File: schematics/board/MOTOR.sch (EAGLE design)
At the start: 77 parts

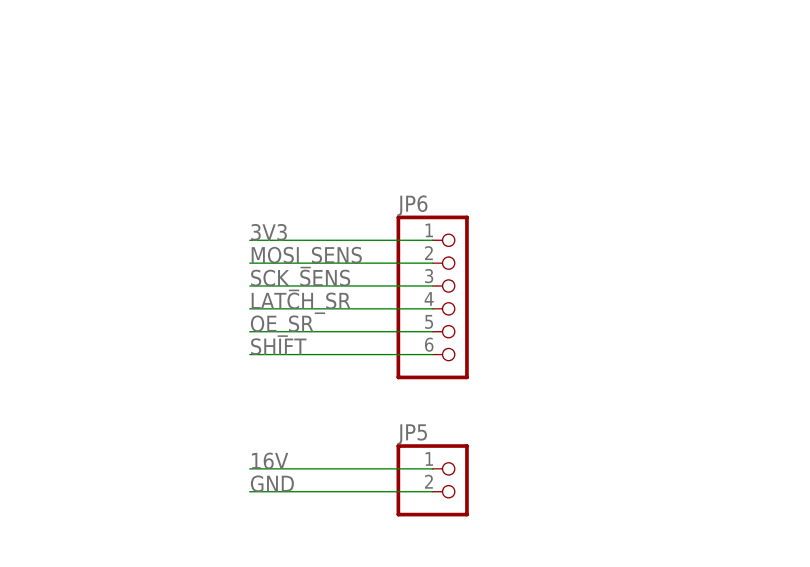
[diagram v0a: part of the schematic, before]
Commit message: Моторчики
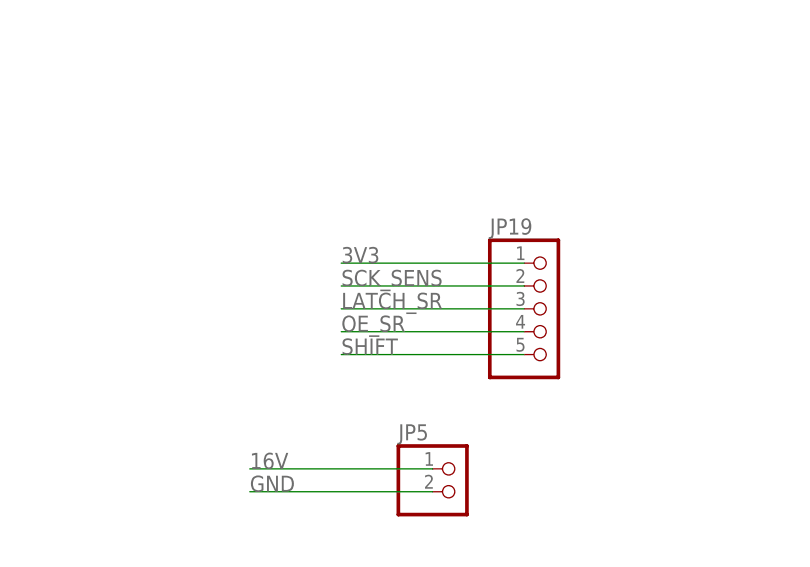
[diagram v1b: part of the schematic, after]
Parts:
- removed JP6: (no value), pinhead:PINHD-1X6
- added JP19: (no value), pinhead:PINHD-1X5
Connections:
- removed net MOSI_SENS: JP6.2
- net 3V3: now also JP19.1; no longer JP6.1
- net LATCH_SR: now also JP19.3; no longer JP6.4
- net OE_SR: now also JP19.4; no longer JP6.5
- net SCK_SENS: now also JP19.2; no longer JP6.3
- net SHIFT: now also JP19.5; no longer JP6.6
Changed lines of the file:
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@@
 <part name="U$2" library="CanCubeSat" deviceset="CONCEVIC" device=""/>
 <part name="JP5" library="pinhead" library_urn="urn:adsk.eagle:library:325" deviceset="PINHD-1X2" device="" package3d_urn="urn:adsk.eagle:package:22435/2"/>
-<part name="JP6" library="pinhead" library_urn="urn:adsk.eagle:library:325" deviceset="PINHD-1X6" device="" package3d_urn="urn:adsk.eagle:package:22472/2"/>
 <part name="SI2302CDS5" library="CanCubeSat" deviceset="SI2302CDS" device=""/>
 <part name="R7" library="rcl" library_urn="urn:adsk.eagle:library:334" deviceset="R-US_" device="R0603" package3d_urn="urn:adsk.eagle:package:23555/3" value="100R"/>
@@
 <part name="U$9" library="UNKNOWN-2024" deviceset="LOGO" device="PCB-&quot;&quot;" value="Плата МОТОРОВ"/>
 <part name="U$10" library="UNKNOWN-2024" deviceset="MOLEX-2-1.25" device=""/>
+<part name="JP19" library="pinhead" library_urn="urn:adsk.eagle:library:325" deviceset="PINHD-1X5" device="" package3d_urn="urn:adsk.eagle:package:22469/2"/>
 </parts>
 <sheets>
@@
 <attribute name="VALUE" x="-21.59" y="38.1" size="1.778" layer="96"/>
 </instance>
-<instance part="JP6" gate="A" x="-15.24" y="63.5" smashed="yes">
-<attribute name="NAME" x="-21.59" y="74.295" size="1.778" layer="95"/>
-<attribute name="VALUE" x="-21.59" y="53.34" size="1.778" layer="96"/>
-</instance>
 <instance part="SI2302CDS5" gate="G$1" x="81.28" y="-30.48" smashed="yes"/>
 <instance part="R7" gate="G$1" x="81.28" y="2.54" smashed="yes" rot="R270">
@@
 <attribute name="VALUE" x="-154.94" y="-39.37" size="1.778" layer="96" rot="R90"/>
 <attribute name="NAME" x="-165.862" y="-39.37" size="1.778" layer="95" rot="R90"/>
+</instance>
+<instance part="JP19" gate="A" x="-5.08" y="63.5" smashed="yes">
+<attribute name="NAME" x="-11.43" y="71.755" size="1.778" layer="95"/>
+<attribute name="VALUE" x="-11.43" y="53.34" size="1.778" layer="96"/>
 </instance>
 </instances>
@@
 </segment>
 <segment>
-<wire x1="-17.78" y1="71.12" x2="-38.1" y2="71.12" width="0.1524" layer="91"/>
-<label x="-38.1" y="71.12" size="1.778" layer="95"/>
-<pinref part="JP6" gate="A" pin="1"/>
+<wire x1="-7.62" y1="68.58" x2="-27.94" y2="68.58" width="0.1524" layer="91"/>
+<label x="-27.94" y="68.58" size="1.778" layer="95"/>
+<pinref part="JP19" gate="A" pin="1"/>
 </segment>
 </net>
@@
 </segment>
 <segment>
-<wire x1="-17.78" y1="60.96" x2="-38.1" y2="60.96" width="0.1524" layer="91"/>
-<label x="-38.1" y="60.96" size="1.778" layer="95"/>
-<pinref part="JP6" gate="A" pin="5"/>
+<wire x1="-7.62" y1="60.96" x2="-27.94" y2="60.96" width="0.1524" layer="91"/>
+<label x="-27.94" y="60.96" size="1.778" layer="95"/>
+<pinref part="JP19" gate="A" pin="4"/>
 </segment>
 </net>
@@
 </segment>
 </net>
-<net name="MOSI_SENS" class="0">
-<segment>
-<wire x1="-17.78" y1="68.58" x2="-38.1" y2="68.58" width="0.1524" layer="91"/>
-<label x="-38.1" y="68.58" size="1.778" layer="95"/>
-<pinref part="JP6" gate="A" pin="2"/>
-</segment>
-</net>
 <net name="SCK_SENS" class="0">
-<segment>
-<wire x1="-17.78" y1="66.04" x2="-38.1" y2="66.04" width="0.1524" layer="91"/>
-<label x="-38.1" y="66.04" size="1.778" layer="95"/>
-<pinref part="JP6" gate="A" pin="3"/>
-</segment>
 <segment>
 <pinref part="U$13" gate="G$1" pin="SHCP"/>
@@
 <label x="68.58" y="58.42" size="1.778" layer="95"/>
 </segment>
+<segment>
+<wire x1="-7.62" y1="66.04" x2="-27.94" y2="66.04" width="0.1524" layer="91"/>
+<label x="-27.94" y="66.04" size="1.778" layer="95"/>
+<pinref part="JP19" gate="A" pin="2"/>
+</segment>
 </net>
 <net name="LATCH_SR" class="0">
-<segment>
-<wire x1="-17.78" y1="63.5" x2="-38.1" y2="63.5" width="0.1524" layer="91"/>
-<label x="-38.1" y="63.5" size="1.778" layer="95"/>
-<pinref part="JP6" gate="A" pin="4"/>
-</segment>
 <segment>
 <pinref part="U$13" gate="G$1" pin="STCP"/>
@@
 <label x="68.58" y="60.96" size="1.778" layer="95"/>
 </segment>
+<segment>
+<wire x1="-7.62" y1="63.5" x2="-27.94" y2="63.5" width="0.1524" layer="91"/>
+<label x="-27.94" y="63.5" size="1.778" layer="95"/>
+<pinref part="JP19" gate="A" pin="3"/>
+</segment>
 </net>
 <net name="SHIFT" class="0">
-<segment>
-<wire x1="-17.78" y1="58.42" x2="-38.1" y2="58.42" width="0.1524" layer="91"/>
-<label x="-38.1" y="58.42" size="1.778" layer="95"/>
-<pinref part="JP6" gate="A" pin="6"/>
-</segment>
 <segment>
 <pinref part="U$13" gate="G$1" pin="DS"/>
@@
 <label x="68.58" y="66.04" size="1.778" layer="95"/>
 </segment>
-</net>
+<segment>
+<wire x1="-7.62" y1="58.42" x2="-27.94" y2="58.42" width="0.1524" layer="91"/>
+<label x="-27.94" y="58.42" size="1.778" layer="95"/>
+<pinref part="JP19" gate="A" pin="5"/>
+</segment>
+</net>

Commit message: Платы готовы
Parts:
- removed JP1, JP11, JP13, JP15, JP17, JP3, JP5, JP7, JP9, MOTOR1, MOTOR2, MOTOR3, MOTOR4, MOTOR5, MOTOR6, MOTOR7: (no value), pinhead:PINHD-1X2
- removed JP10, JP12, JP14, JP16, JP18, JP2, JP4, JP8: (no value), pinhead:PINHD-1X3
- removed JP19: (no value), pinhead:PINHD-1X5
- removed SI2302CDS1, SI2302CDS10, SI2302CDS11, SI2302CDS12, SI2302CDS13, SI2302CDS14, SI2302CDS15, SI2302CDS16, SI2302CDS2, SI2302CDS3, SI2302CDS4, SI2302CDS5, SI2302CDS6, SI2302CDS7, SI2302CDS8, SI2302CDS9: SI2302CDS, CanCubeSat:SI2302CDS
- removed U$1, U$2, U$3, U$4, U$6, U$7, U$8: CONCEVIC, CanCubeSat:CONCEVIC
- added 16V, GND: (no value), pinhead:PINHD-1X2/90
- added BUT0, BUT1, BUT2, BUT3, BUT4, BUT5, BUT6, BUT7: (no value), pinheadCS:PINHD-1X2
- added END0, END1, END2, END3, END4, END5, END6, END7: CONCEVIC, CanCubeSat:CONCEVIC
- added MOT0, MOT1, MOT2, MOT3, MOT4, MOT5, MOT6, MOT7, PWR_16V: JST-2-2.5, UNKNOWN-2024:JST-2-2.5
- added RADIO: MOLEX-5-1.25, UNKNOWN-2024:MOLEX-5-1.25
- added U$11, U$15, U$16, U$20, U$28, U$32: IRF5852, NA-2025:IRF5852
- added U$35, U$36, U$37, U$38, U$39, U$40, U$41, U$42: CONTACT_SIDE_4MM_2PIN, UNKNOWN-2024:CONTACT_SIDE_4MM_2PIN
- U$10: value MOLEX-2-1.25 -> IRF5852; device UNKNOWN-2024:MOLEX-2-1.25 -> NA-2025:IRF5852
- U$5: value CONCEVIC -> IRF5852; device CanCubeSat:CONCEVIC -> NA-2025:IRF5852
- U$9: value Плата МОТОРОВ -> Плата Моторов
- renumbered U$13 to 74HC595
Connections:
- removed net 16V: JP1.2, JP10.3, JP11.2, JP12.3, JP13.2, JP14.3, JP15.2, JP16.3, JP17.2, JP18.3, JP2.3, JP3.2, JP4.3, JP5.1, JP7.2, JP8.3, JP9.2, R12.1, R16.1, R19.1, R22.1, R25.1, R3.1, R6.1, R9.1
- removed net GND: 74HC595.GND, JP5.2, R11.2, R14.1, R15.2, R18.2, R2.2, R21.2, R24.2, R5.2, R8.2, SI2302CDS1.S, SI2302CDS10.S, SI2302CDS11.S, SI2302CDS12.S, SI2302CDS13.S, SI2302CDS14.S, SI2302CDS15.S, SI2302CDS16.S, SI2302CDS2.S, SI2302CDS3.S, SI2302CDS4.S, SI2302CDS5.S, SI2302CDS6.S, SI2302CDS7.S, SI2302CDS8.S, SI2302CDS9.S, U$1.P, U$2.P, U$3.P, U$4.P, U$5.P, U$6.P, U$7.P, U$8.P
- removed net N$33: JP16.2, MOTOR6.1
- removed net N$34: JP16.1, SI2302CDS14.D
- removed net N$35: R22.2, SI2302CDS14.G
- removed net N$36: JP17.1, MOTOR7.2, SI2302CDS15.D
- removed net N$37: R23.2, R24.1, SI2302CDS15.G, U$8.S
- removed net N$38: JP18.2, MOTOR7.1
- removed net N$39: JP18.1, SI2302CDS16.D
- removed net N$40: R25.2, SI2302CDS16.G
- new net 16V_IN: 16V.1, MOT0.1, MOT1.1, MOT2.1, MOT3.1, MOT4.1, MOT5.1, MOT6.1, MOT7.1, U$10G$1.D1, U$11G$1.D1, U$15G$1.D1, U$16G$1.D1, U$20G$1.D1, U$28G$1.D1, U$32G$1.D1, U$5G$1.D1
- new net 16V_OUT: 16V.2, PWR_16V.1
- new net GND_IN: END0.P, END1.P, END2.P, END3.P, END4.P, END5.P, END6.P, END7.P, GND.1, R11.2, R15.2, R18.2, R2.2, R21.2, R24.2, R5.2, R8.2, U$10G$2.S1, U$11G$2.S1, U$15G$2.S1, U$16G$2.S1, U$20G$2.S1, U$28G$2.S1, U$32G$2.S1, U$5G$2.S1
- new net GND_OUT: 74HC595.GND, GND.2, PWR_16V.2, R14.1
- net 3V3: now also RADIO.1; no longer JP19.1
- net LATCH_SR: now also RADIO.3; no longer JP19.3
- net MOTOR0: now also 74HC595.Q7; no longer 74HC595.Q0
- net MOTOR4: now also 74HC595.Q0; no longer 74HC595.Q4
- net MOTOR5: now also 74HC595.Q4; no longer 74HC595.Q5
- net MOTOR6: now also 74HC595.Q5; no longer 74HC595.Q6
- net MOTOR7: now also 74HC595.Q6; no longer 74HC595.Q7
- net N$1: now also MOT0.2, R3.1, U$11G$2.D1, U$38.P$1; no longer JP1.1, SI2302CDS1.D, U$10.2
- net N$10: now also BUT2.2, U$16G$1.S1, U$36.P$2; no longer R6.2, SI2302CDS4.G
- net N$11: now also END3.S, R10.2, R11.1, U$5G$2.G1; no longer JP7.1, MOTOR2.2, SI2302CDS5.D
- net N$12: now also END2.S, U$16G$2.G1; no longer SI2302CDS5.G, U$3.S
- net N$13: now also BUT2.1, R9.1, U$16G$1.G1; no longer JP8.2, MOTOR2.1
- net N$14: now also MOT3.2, R12.2, U$37.P$1, U$5G$2.D1; no longer JP8.1, SI2302CDS6.D
- net N$15: now also BUT3.2, U$37.P$2, U$5G$1.S1; no longer R9.2, SI2302CDS6.G
- net N$16: now also BUT3.1, R12.1, U$5G$1.G1; no longer JP9.1, MOTOR3.2, SI2302CDS7.D
- net N$17: now also END4.S, R13.2, R15.1, U$15G$2.G1; no longer R10.2, R11.1, SI2302CDS7.G, U$4.S
- net N$18: now also MOT4.2, R16.2, U$15G$2.D1, U$39.P$1; no longer JP10.2, MOTOR3.1
- net N$19: now also BUT4.2, U$15G$1.S1, U$39.P$2; no longer JP10.1, SI2302CDS8.D
- net N$2: now also MOT1.2, R6.2, U$10G$2.D1, U$35.P$1; no longer JP3.1, MOTOR1.2, SI2302CDS3.D
- net N$20: now also BUT4.1, R16.1, U$15G$1.G1; no longer R12.2, SI2302CDS8.G
- net N$21: now also END5.S, R17.2, R18.1, U$20G$2.G1; no longer JP11.1, MOTOR4.2, SI2302CDS9.D
- net N$22: now also MOT5.2, R19.2, U$20G$2.D1, U$40.P$1; no longer R13.2, R15.1, SI2302CDS9.G, U$5.S
- net N$23: now also BUT5.2, U$20G$1.S1, U$40.P$2; no longer JP12.2, MOTOR4.1
- net N$24: now also BUT5.1, R19.1, U$20G$1.G1; no longer JP12.1, SI2302CDS10.D
- net N$25: now also END6.S, R20.2, R21.1, U$28G$2.G1; no longer R16.2, SI2302CDS10.G
- net N$26: now also MOT6.2, R22.2, U$28G$2.D1, U$41.P$1; no longer JP13.1, MOTOR5.2, SI2302CDS11.D
- net N$27: now also BUT6.2, U$28G$1.S1, U$41.P$2; no longer R17.2, R18.1, SI2302CDS11.G, U$6.S
- net N$28: now also BUT6.1, R22.1, U$28G$1.G1; no longer JP14.2, MOTOR5.1
- net N$29: now also END7.S, R23.2, R24.1, U$32G$2.G1; no longer JP14.1, SI2302CDS12.D
- net N$3: now also END1.S, U$10G$2.G1; no longer SI2302CDS3.G, U$2.S
- net N$30: now also MOT7.2, R25.2, U$32G$2.D1, U$42.P$1; no longer R19.2, SI2302CDS12.G
- net N$31: now also BUT7.2, U$32G$1.S1, U$42.P$2; no longer JP15.1, MOTOR6.2, SI2302CDS13.D
- net N$32: now also BUT7.1, R25.1, U$32G$1.G1; no longer R20.2, R21.1, SI2302CDS13.G, U$7.S
- net N$4: now also END0.S, U$11G$2.G1; no longer SI2302CDS1.G, U$1.S
- net N$5: now also BUT1.2, U$10G$1.S1, U$35.P$2; no longer JP4.2, MOTOR1.1
- net N$6: now also BUT0.1, R3.2, U$11G$1.G1; no longer JP2.2, U$10.1
- net N$7: now also BUT1.1, R6.1, U$10G$1.G1; no longer JP4.1, SI2302CDS4.D
- net N$8: now also BUT0.2, U$11G$1.S1, U$38.P$2; no longer JP2.1, SI2302CDS2.D
- net N$9: now also MOT2.2, R9.2, U$16G$2.D1, U$36.P$1; no longer R3.2, SI2302CDS2.G
- net OE_SR: now also RADIO.4; no longer JP19.4
- net SCK_SENS: now also RADIO.2; no longer JP19.2
- net SHIFT: now also RADIO.5; no longer JP19.5
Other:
- moved on the sheet: R1, R10, R11, R12, R13, R15, R16, R17, R18, R19, R20, R21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
